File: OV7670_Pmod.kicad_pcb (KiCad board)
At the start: 2 copper layers, 27.1 x 39.5 mm, 7 parts, among them U1 Pmod_connector, U2 Pmod_connector, U3 OV7670_camera

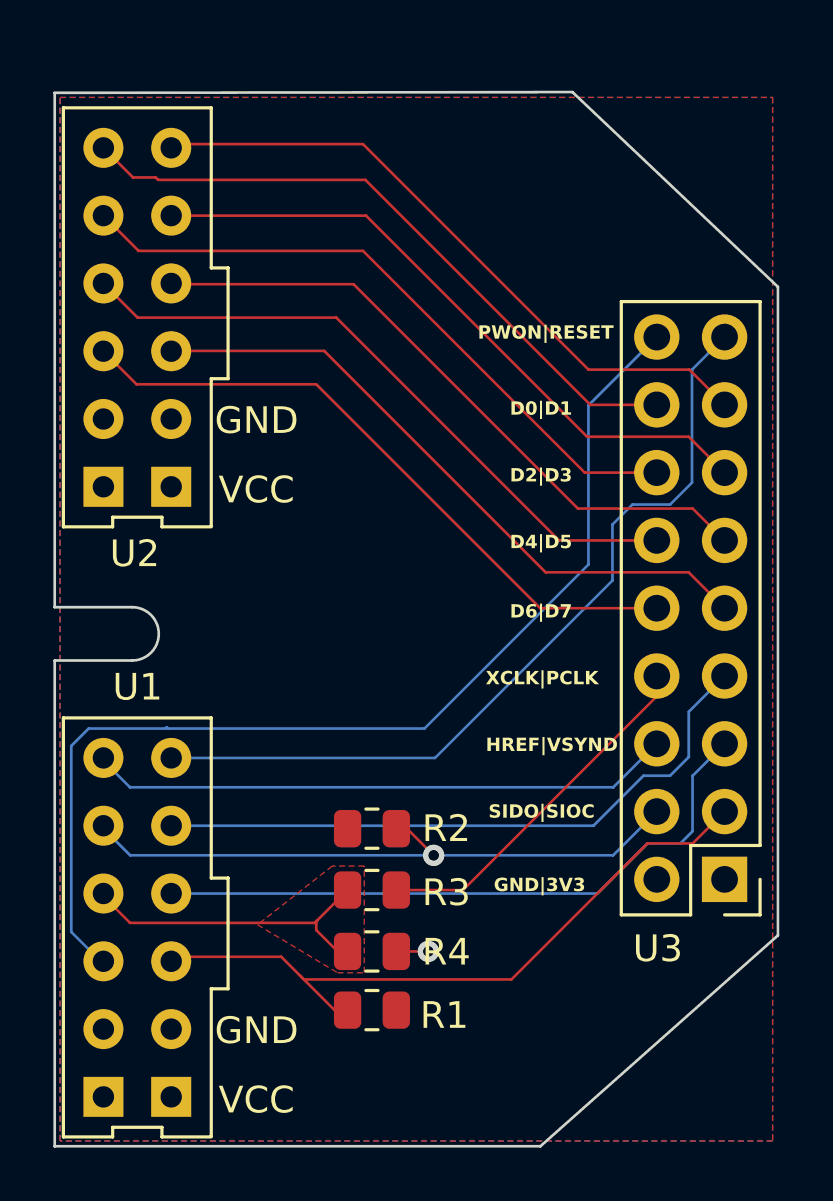
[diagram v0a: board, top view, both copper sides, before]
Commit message: update
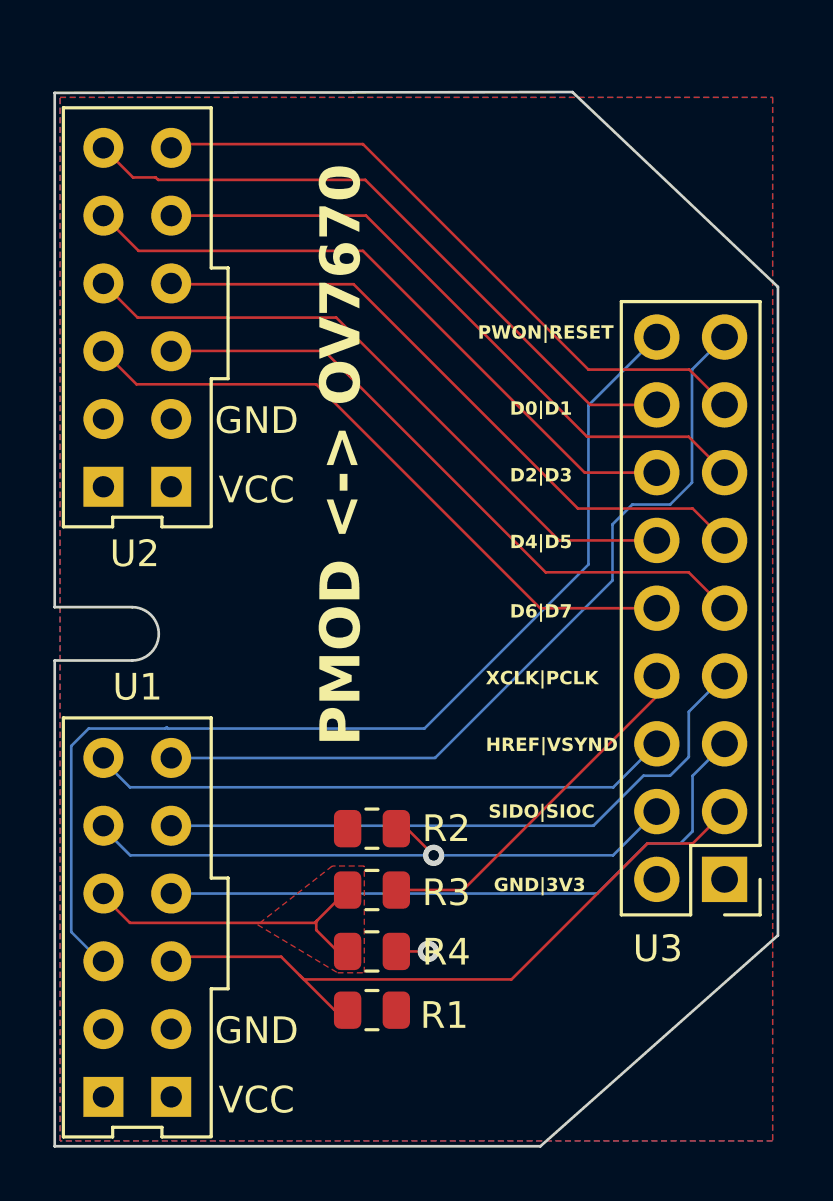
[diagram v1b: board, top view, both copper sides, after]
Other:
- board text added: "PMOD <-> OV7670"
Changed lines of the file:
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@@
         (effects (font (size 1 1) (thickness 0.15)))
+    )
+    (fp_text user "PWON|RESET" (at -8 -10.15 unlocked) (layer "F.SilkS")
+        (effects (font (size 0.5 0.5) (thickness 0.1) bold) (justify left bottom))
     )
     (fp_text user "D4|D5" (at -6.8 -2.3 unlocked) (layer "F.SilkS")
         (effects (font (size 0.5 0.5) (thickness 0.1) bold) (justify left bottom))
     )
+    (fp_text user "D6|D7" (at -6.8 0.3 unlocked) (layer "F.SilkS")
+        (effects (font (size 0.5 0.5) (thickness 0.1) bold) (justify left bottom))
+    )
+    (fp_text user "SIDO|SIOC" (at -7.6 7.8 unlocked) (layer "F.SilkS")
+        (effects (font (size 0.5 0.5) (thickness 0.1) bold) (justify left bottom))
+    )
+    (fp_text user "HREF|VSYND" (at -7.7 5.3 unlocked) (layer "F.SilkS")
+        (effects (font (size 0.5 0.5) (thickness 0.1) bold) (justify left bottom))
+    )
+    (fp_text user "D2|D3" (at -6.8 -4.8 unlocked) (layer "F.SilkS")
+        (effects (font (size 0.5 0.5) (thickness 0.1) bold) (justify left bottom))
+    )
+    (fp_text user "D0|D1" (at -6.8 -7.3 unlocked) (layer "F.SilkS")
+        (effects (font (size 0.5 0.5) (thickness 0.1) bold) (justify left bottom))
+    )
     (fp_text user "GND|3V3" (at -7.4 10.55 unlocked) (layer "F.SilkS")
         (effects (font (size 0.5 0.5) (thickness 0.1) bold) (justify left bottom))
     )
-    (fp_text user "PWON|RESET" (at -8 -10.15 unlocked) (layer "F.SilkS")
-        (effects (font (size 0.5 0.5) (thickness 0.1) bold) (justify left bottom))
-    )
-    (fp_text user "HREF|VSYND" (at -7.7 5.3 unlocked) (layer "F.SilkS")
-        (effects (font (size 0.5 0.5) (thickness 0.1) bold) (justify left bottom))
-    )
-    (fp_text user "D6|D7" (at -6.8 0.3 unlocked) (layer "F.SilkS")
-        (effects (font (size 0.5 0.5) (thickness 0.1) bold) (justify left bottom))
-    )
-    (fp_text user "D2|D3" (at -6.8 -4.8 unlocked) (layer "F.SilkS")
-        (effects (font (size 0.5 0.5) (thickness 0.1) bold) (justify left bottom))
-    )
-    (fp_text user "D0|D1" (at -6.8 -7.3 unlocked) (layer "F.SilkS")
-        (effects (font (size 0.5 0.5) (thickness 0.1) bold) (justify left bottom))
-    )
     (fp_text user "XCLK|PCLK" (at -7.7 2.8 unlocked) (layer "F.SilkS")
-        (effects (font (size 0.5 0.5) (thickness 0.1) bold) (justify left bottom))
-    )
-    (fp_text user "SIDO|SIOC" (at -7.6 7.8 unlocked) (layer "F.SilkS")
         (effects (font (size 0.5 0.5) (thickness 0.1) bold) (justify left bottom))
     )
@@
     (pad "18" thru_hole oval locked (at -1.29 -10.27 180) (size 1.7 1.7) (drill 1) (layers "*.Cu" "*.Mask")
       (net 11 "/PWON") (pinfunction "PWON") (pintype "input"))
+    (model ":KICAD7_3DMODEL_DIR:Connector_PinHeader_2.54mm.3dshapes/PinHeader_2x09_P2.54mm_Horizontal.step"
+      (offset (xyz -1.25 10.25 0))
+      (scale (xyz 1 1 1))
+      (rotate (xyz 0 0 0))
+    )
   )
   (footprint "Resistor_SMD:R_0805_2012Metric" (layer "F.Cu")
@@
         (effects (font (size 1 1) (thickness 0.15)))
     )
+    (fp_text user "GND" (at 3.8 -4.2 unlocked) (layer "F.SilkS")
+        (effects (font (size 1 1) (thickness 0.15)))
+    )
     (fp_text user "VCC" (at 6.4 -4.2 unlocked) (layer "F.SilkS")
-        (effects (font (size 1 1) (thickness 0.15)))
-    )
-    (fp_text user "GND" (at 3.8 -4.2 unlocked) (layer "F.SilkS")
         (effects (font (size 1 1) (thickness 0.15)))
     )
@@
     (pad "12" thru_hole rect locked (at 6.28 1.54 90) (size 1.5 1.5) (drill 0.8) (layers "*.Cu" "*.Mask")
       (net 2 "+3V3") (pinfunction "VCC") (pintype "power_in"))
+    (model ":KICAD7_3DMODEL_DIR:Connector_PinHeader_2.54mm.3dshapes/PinHeader_2x06_P2.54mm_Horizontal.step"
+      (offset (xyz 6.25 1 0))
+      (scale (xyz 1 1 1))
+      (rotate (xyz 0 0 90))
+    )
   )
   (footprint "Resistor_SMD:R_0805_2012Metric" (layer "F.Cu")
@@
         (effects (font (size 1 1) (thickness 0.15)))
     )
+    (fp_text user "GND" (at 3.8 -4.2 unlocked) (layer "F.SilkS")
+        (effects (font (size 1 1) (thickness 0.15)))
+    )
     (fp_text user "VCC" (at 6.4 -4.2 unlocked) (layer "F.SilkS")
-        (effects (font (size 1 1) (thickness 0.15)))
-    )
-    (fp_text user "GND" (at 3.8 -4.2 unlocked) (layer "F.SilkS")
         (effects (font (size 1 1) (thickness 0.15)))
     )
@@
     (pad "12" thru_hole rect locked (at 6.28 1.54 90) (size 1.5 1.5) (drill 0.8) (layers "*.Cu" "*.Mask")
       (net 2 "+3V3") (pinfunction "VCC") (pintype "power_in"))
+    (model ":KICAD7_3DMODEL_DIR:Connector_PinHeader_2.54mm.3dshapes/PinHeader_2x06_P2.54mm_Horizontal.step"
+      (offset (xyz 6.25 1 0))
+      (scale (xyz 1 1 1))
+      (rotate (xyz 0 0 90))
+    )
   )
   (gr_line (start 104.3 80.1) (end 104.3 104.4)
@@
   (gr_line (start 77.2 112.3) (end 95.4 112.3)
     (stroke (width 0.1) (type default)) (layer "Edge.Cuts"))
+  (gr_text "PMOD <-> OV7670" (at 88.8 97.3 90) (layer "F.SilkS")
+    (effects (font (size 1.5 1.5) (thickness 0.3) bold) (justify left bottom))
+  )
   (segment (start 86.3875 105.9) (end 86.5375 106.05) (width 0.1) (layer "F.Cu") (net 1))
   (segment (start 85.6875 105.2) (end 86.3875 105.9) (width 0.1) (layer "F.Cu") (net 1))
